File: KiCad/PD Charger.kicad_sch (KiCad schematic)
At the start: 106 parts, among them J1 USB_C_Receptacle_USB2.0, J2 Conn_ARM_SWD_TagConnect_TC2030, J3 XT60_M, Q1 NMOS, Q2 NMOS, Q3 NMOS, Q4 NMOS, Q5 NTMFS002P03, Q6 NTMFS002P03, Q7 Q_Dual_NMOS_S1G1D2S2G2D1, Q8 Q_Dual_NMOS_S1G1D2S2G2D1, SW1 SW_MEC_5G, SW2 SW_MEC_5G, U1 FUSB302B01MPX, U2 LMR36006BRNXT, U3 LT8390xFE, U4 STM32G431CBUx

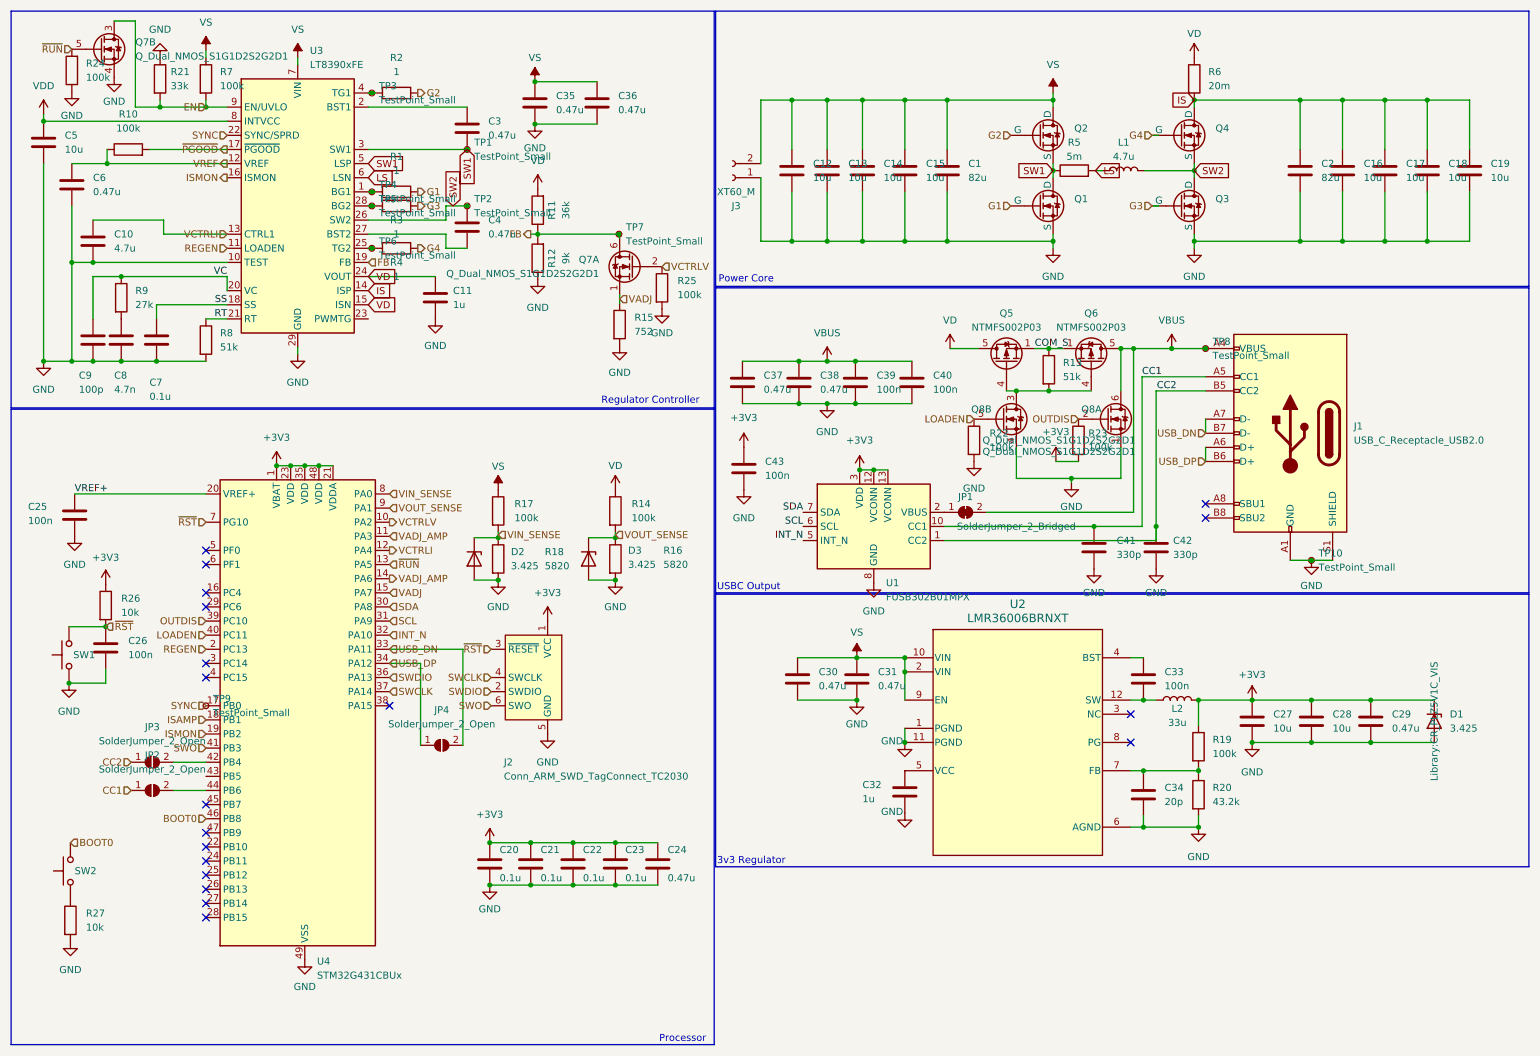
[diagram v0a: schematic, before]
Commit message: multisheet design
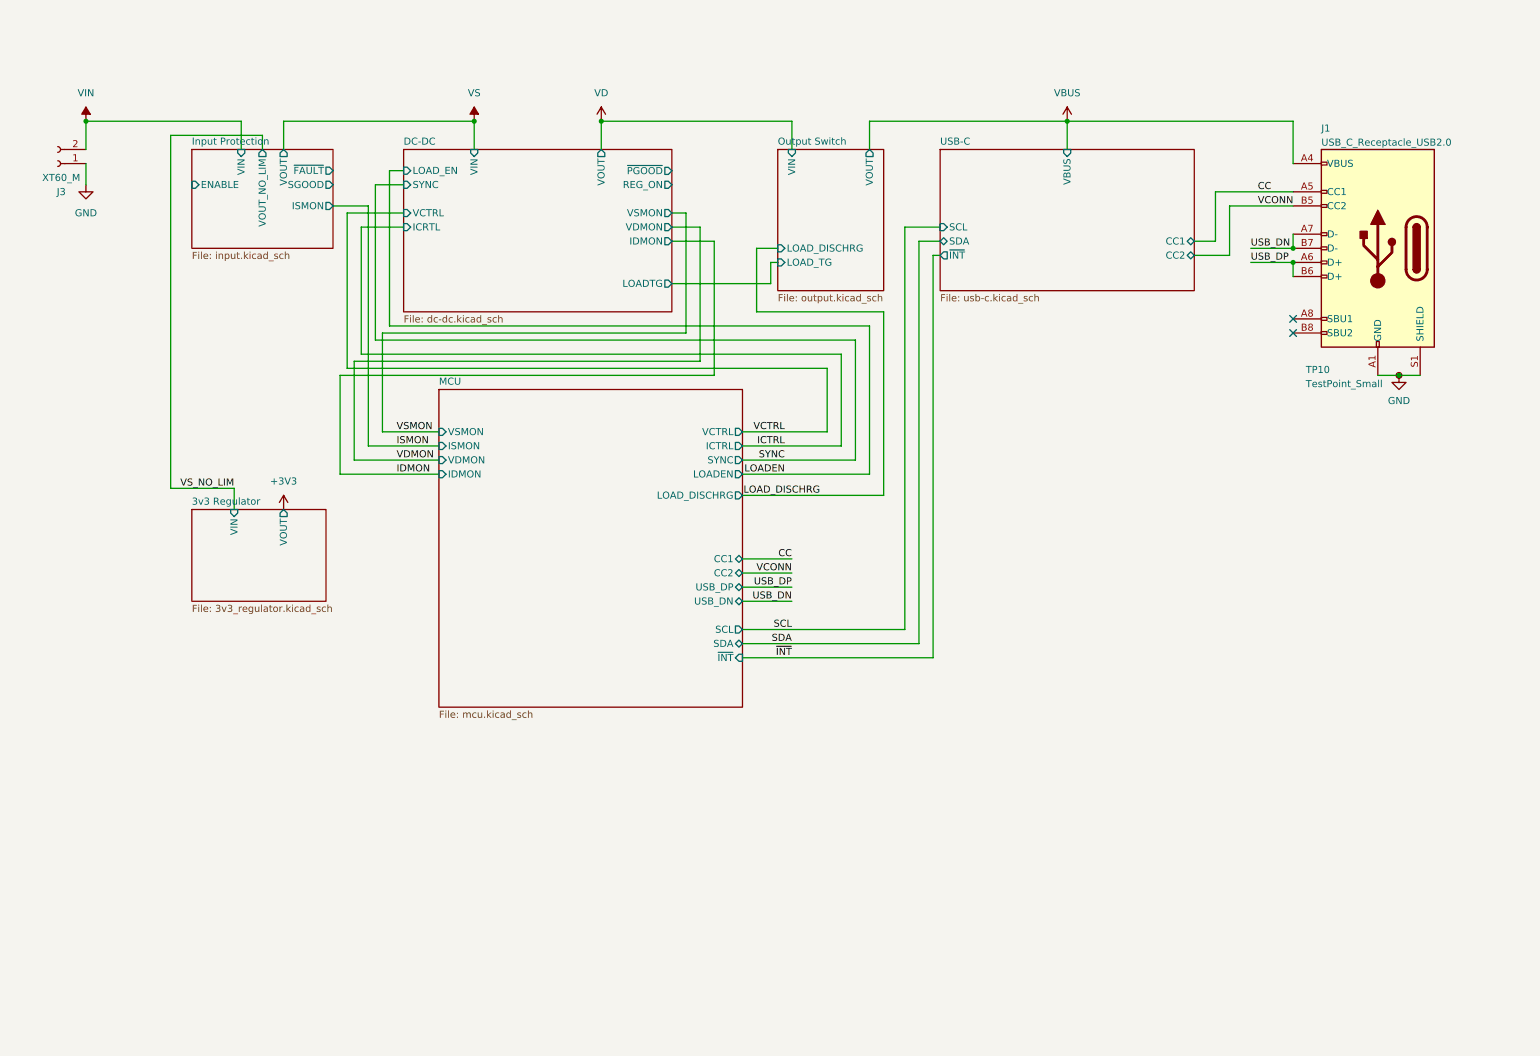
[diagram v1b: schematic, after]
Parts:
- removed C1, C2: 82u, Capacitor_SMD:CP_Elec_10x7.9, symbol Device:C
- removed C10: 4.7u, Capacitor_SMD:C_0603_1608Metric, symbol Device:C
- removed C11, C32: 1u, Capacitor_SMD:C_0603_1608Metric, symbol Device:C
- removed C12, C13, C14, C15, C16, C17, C18, C19, C27, C28, C5: 10u, Capacitor_SMD:C_1206_3216Metric, symbol Device:C
- removed C20, C21, C22, C23, C7: 0.1u, Capacitor_SMD:C_0603_1608Metric, symbol Device:C
- removed C24, C6: 0.47u, Capacitor_SMD:C_0603_1608Metric, symbol Device:C
- removed C25, C26, C33, C39, C40, C43: 100n, Capacitor_SMD:C_0603_1608Metric, symbol Device:C
- removed C29, C3, C30, C31, C35, C36, C37, C38, C4: 0.47u, Capacitor_SMD:C_0805_2012Metric, symbol Device:C
- removed C34: 20p, Capacitor_SMD:C_0603_1608Metric, symbol Device:C
- removed C41, C42: 330p, Capacitor_SMD:C_0603_1608Metric, symbol Device:C
- removed C8: 4.7n, Capacitor_SMD:C_0603_1608Metric, symbol Device:C
- removed C9: 100p, Capacitor_SMD:C_0603_1608Metric, symbol Device:C
- removed D1, D2, D3: 3.425, Library:CR_PLZ5V1C_VIS, symbol Device:D_Zener
- removed J2: Conn_ARM_SWD_TagConnect_TC2030, Connector:Tag-Connect_TC2030-IDC-NL_2x03_P1.27mm_Vertical, symbol Connector:Conn_ARM_SWD_TagConnect_TC2030
- removed JP1: SolderJumper_2_Bridged, Jumper:SolderJumper-2_P1.3mm_Bridged2Bar_RoundedPad1.0x1.5mm, symbol Jumper:SolderJumper_2_Bridged
- removed JP2, JP3, JP4: SolderJumper_2_Open, Jumper:SolderJumper-2_P1.3mm_Open_RoundedPad1.0x1.5mm, symbol Jumper:SolderJumper_2_Open
- removed L1: 4.7u, Inductor_SMD:L_Vishay_IHLP-6767, symbol Device:L
- removed L2: 33u, Inductor_SMD:L_Wuerth_MAPI-3015, symbol Device:L
- removed Q1, Q2, Q3, Q4: NMOS, Library:ECP2302, symbol Simulation_SPICE:NMOS
- removed Q5, Q6: NTMFS002P03, Package_DFN_QFN:AO_DFN-8-1EP_5.55x5.2mm_P1.27mm_EP4.12x4.6mm, symbol Transistor_FET:AON6411
- removed Q7, Q8: Q_Dual_NMOS_S1G1D2S2G2D1, Package_TO_SOT_SMD:SOT-363_SC-70-6, symbol Device:Q_Dual_NMOS_S1G1D2S2G2D1
- removed R1, R2, R3, R4: 1, Resistor_SMD:R_0603_1608Metric, symbol Device:R
- removed R10, R14, R17, R19, R22, R23, R24, R25, R7: 100k, Resistor_SMD:R_0603_1608Metric, symbol Device:R
- removed R11: 36k, Resistor_SMD:R_0603_1608Metric, symbol Device:R
- removed R12: 9k, Resistor_SMD:R_0603_1608Metric, symbol Device:R
- removed R13, R8: 51k, Resistor_SMD:R_0603_1608Metric, symbol Device:R
- removed R15: 752, Resistor_SMD:R_0603_1608Metric, symbol Device:R
- removed R16, R18: 5820, Resistor_SMD:R_0603_1608Metric, symbol Device:R
- removed R20: 43.2k, Resistor_SMD:R_0603_1608Metric, symbol Device:R
- removed R21: 33k, Resistor_SMD:R_0603_1608Metric, symbol Device:R
- removed R26, R27: 10k, Resistor_SMD:R_0603_1608Metric, symbol Device:R
- removed R5: 5m, Resistor_SMD:R_1206_3216Metric, symbol Device:R
- removed R6: 20m, Resistor_SMD:R_1206_3216Metric, symbol Device:R
- removed R9: 27k, Resistor_SMD:R_0603_1608Metric, symbol Device:R
- removed SW1, SW2: SW_MEC_5G, Button_Switch_SMD:SW_SPST_B3U-1000P-B, symbol Switch:SW_Push
- removed TP1, TP2, TP3, TP4, TP5, TP6, TP7, TP8, TP9: TestPoint_Small, TestPoint:TestPoint_Pad_D1.0mm, symbol Connector:TestPoint_Small
- removed U1: FUSB302B01MPX, Package_DFN_QFN:WQFN-14-1EP_2.5x2.5mm_P0.5mm_EP1.45x1.45mm, symbol Interface_USB:FUSB302B01MPX
- removed U2: LMR36006BRNXT, Library:RNX0012B, symbol 2024-04-12_02-42-06:LMR36006BRNXT
- removed U3: LT8390xFE, Package_SO:TSSOP-28-1EP_4.4x9.7mm_P0.65mm, symbol Driver_LED:LT8391xFE
- removed U4: STM32G431CBUx, Package_DFN_QFN:QFN-48-1EP_7x7mm_P0.5mm_EP5.6x5.6mm, symbol MCU_ST_STM32G4:STM32G431C6Ux
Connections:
- net VS: no longer J3.2 (Pin_2)
- net CC1 renamed CC
- net CC2 renamed VCONN
- new net VIN: J3.2 (Pin_2)
- no-connect marks 19 -> 2
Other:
- added sheet 3v3 Regulator (3v3_regulator.kicad_sch)
- added sheet DC-DC (dc-dc.kicad_sch)
- added sheet Input Protection (input.kicad_sch)
- added sheet MCU (mcu.kicad_sch)
- added sheet Output Switch (output.kicad_sch)
- added sheet USB-C (usb-c.kicad_sch)
- note removed: "3v3 Regulator"
- note removed: "Power Core"
- note removed: "Processor"
- note removed: "Regulator Controller"
- note removed: "USBC Output"
- moved on the sheet: J1, J3, TP10
